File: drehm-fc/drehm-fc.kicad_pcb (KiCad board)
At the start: 2 copper layers, 40.5 x 50.5 mm, 16 parts, among them J1 TSW-113-08-T-T-RA, J4 Conn_01x04, U1 DEV-15583

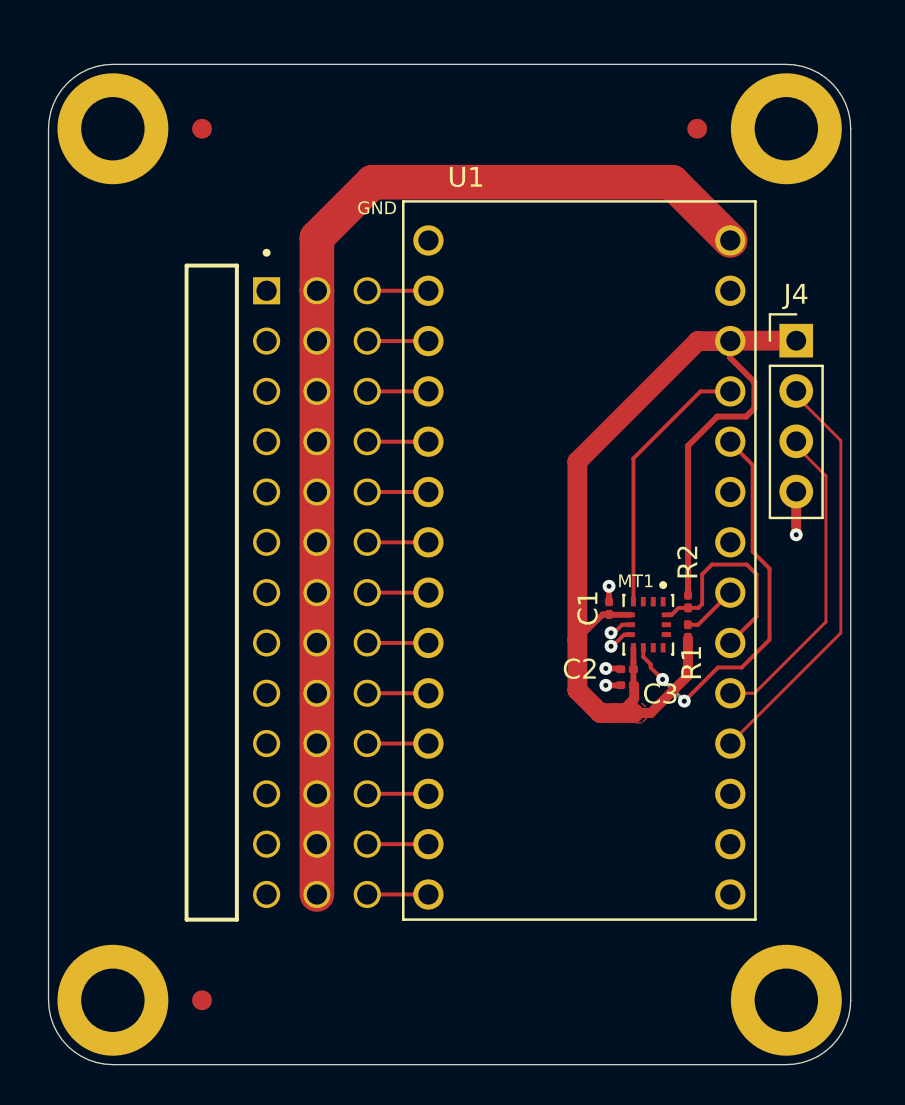
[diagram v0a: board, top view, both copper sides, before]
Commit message: Routing mostly done, finishing touches WIP
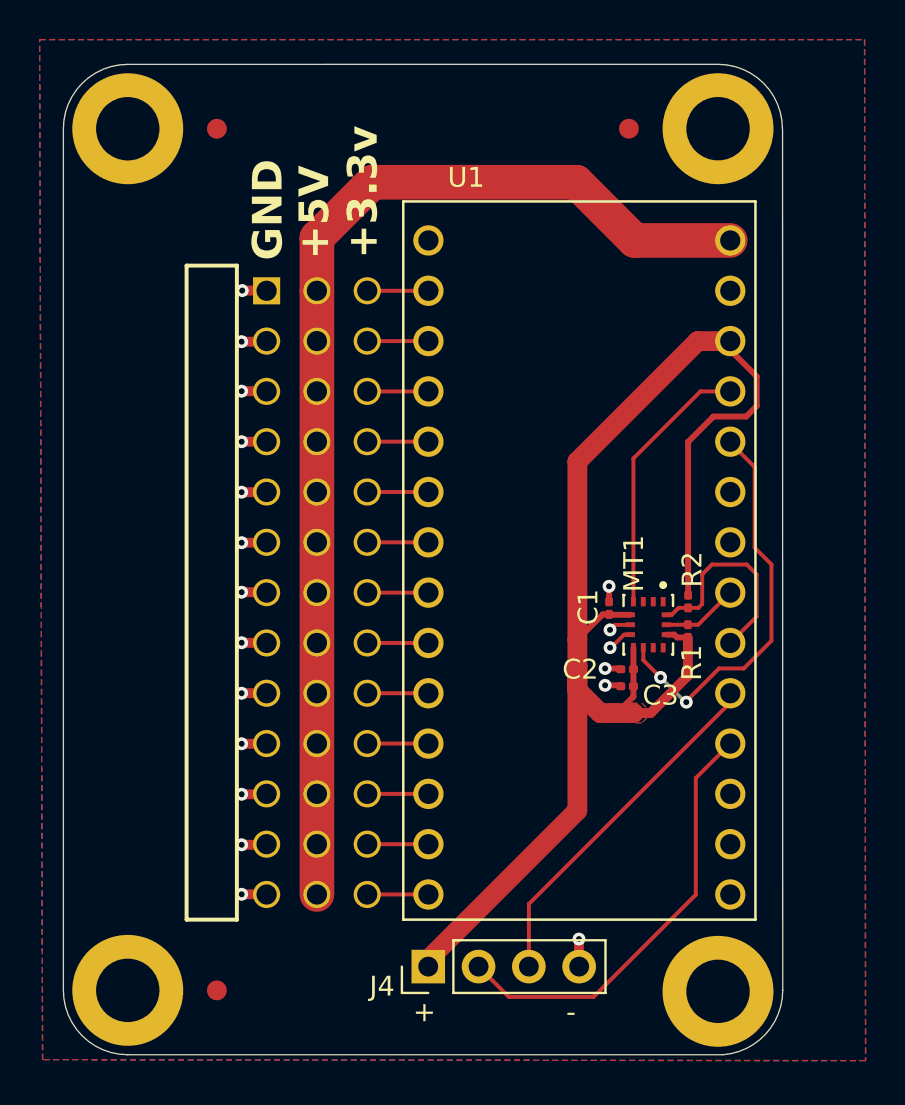
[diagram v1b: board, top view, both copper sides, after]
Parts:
- moved J4 36.7 mm to (140.9, 145.3), turned to 90 degrees
- moved H3 3.48 mm to (155.6, 146.6)
- moved FID2 3.45 mm to (151.1, 103.0)
- moved H2 3.45 mm to (155.6, 103.0)
- moved FID1 0.90 mm to (130.2, 146.5)
- moved H1 0.90 mm to (125.8, 146.5)
- moved FID3 0.75 mm to (130.2, 103.0)
- moved H4 0.75 mm to (125.8, 103.0)
- moved C3 0.06 mm to (151.0, 131.2)
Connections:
- J1 pad 01: Net-(J1-Pad01) -> Earth
- J1 pad 04: Net-(J1-Pad01) -> Earth
- J1 pad 07: Net-(J1-Pad01) -> Earth
- J1 pad 10: Net-(J1-Pad01) -> Earth
- J1 pad 13: Net-(J1-Pad01) -> Earth
- J1 pad 16: Net-(J1-Pad01) -> Earth
- J1 pad 19: Net-(J1-Pad01) -> Earth
- J1 pad 22: Net-(J1-Pad01) -> Earth
- J1 pad 25: Net-(J1-Pad01) -> Earth
- J1 pad 28: Net-(J1-Pad01) -> Earth
- J1 pad 31: Net-(J1-Pad01) -> Earth
- J1 pad 34: Net-(J1-Pad01) -> Earth
- J1 pad 37: Net-(J1-Pad01) -> Earth
- U1 pad G1: Net-(J1-Pad01) -> Earth
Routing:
- net +3V3: track 56.3 -> 73.1 mm
- net Earth: track 6.84 -> 22.8 mm, vias 6 -> 19
- net /UART TX/I2C SDA: track 16.2 -> 18.0 mm
- net /IMU_SCL: track 2.81 -> 3.90 mm
- net /UART RX/I2C SCL: track 21.1 -> 22.1 mm
- added copper zone on B.Cu, net Earth
- added copper zone on F.Cu, net Earth
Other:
- board size 40.5 x 50.5 mm -> 36.3 x 50 mm
- board text added: "+"
- board text added: "+3.3v"
- board text added: "+5V"
- board text added: "-"
- board text added: "GND"
